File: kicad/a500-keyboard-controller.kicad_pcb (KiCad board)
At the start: 2 copper layers, 168 x 39.5 mm, 41 parts, among them J1 ICSP, J2 keyboard_matrix, J3 Mainboard, J4 EARTH_STRAP, Q1 BC557, Q2 BC557, U1 PIC18F4520

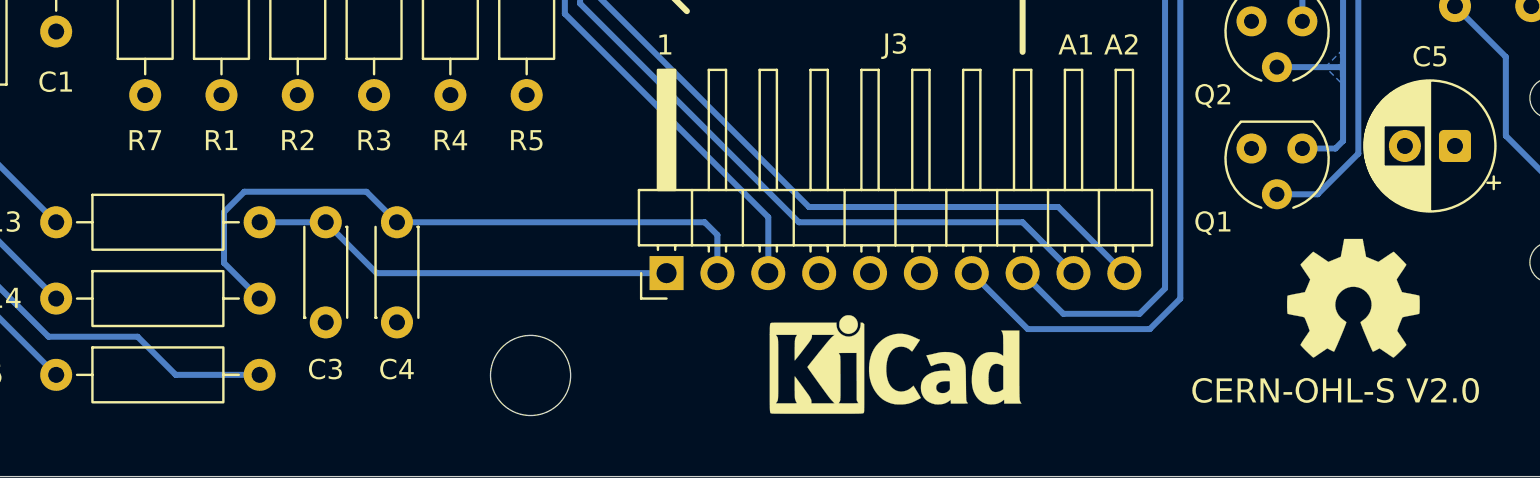
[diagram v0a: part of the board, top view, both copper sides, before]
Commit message: moved OSHW logo a bit, this version sent to fabrication
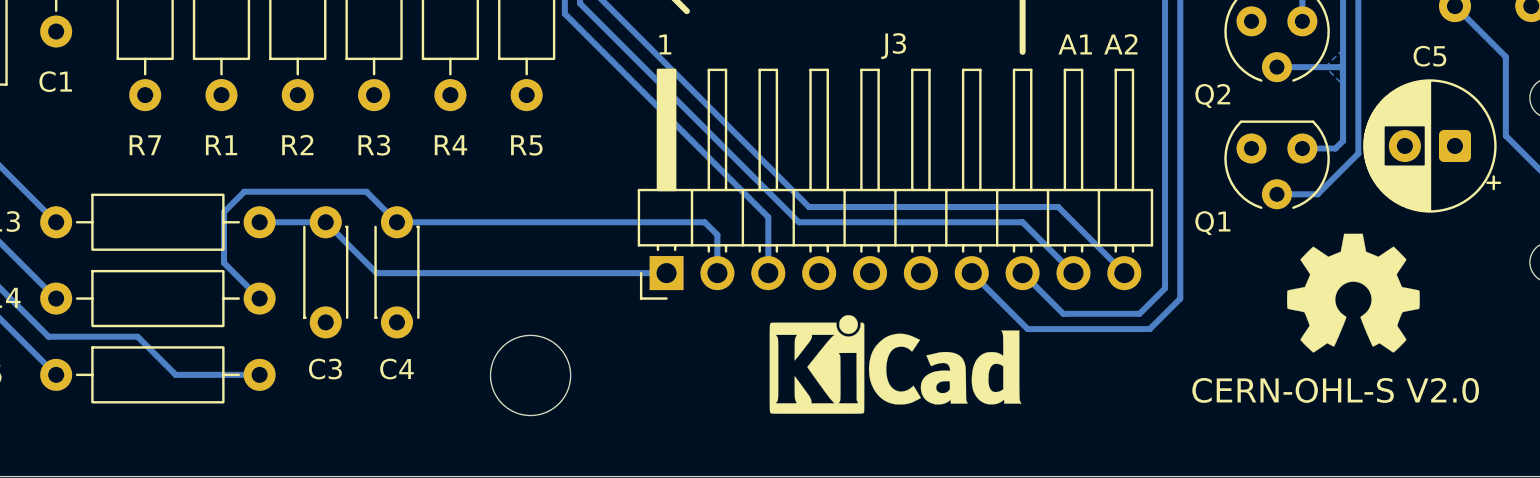
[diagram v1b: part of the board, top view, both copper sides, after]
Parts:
- moved REF2 0.25 mm to (204.5, 114.3)
